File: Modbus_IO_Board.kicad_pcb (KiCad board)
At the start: 2 copper layers, 71.5 x 45 mm, 74 parts, among them IC1 ATMEGA328PB-AN, IC2 TPS7B6933QDCYRQ1, IC3 MAX3072EASA+, IC4 SN74LVC2G14DBVRG4, IC5 LTV-206, J1 Conn_01x06_Male, J2 2.54mm pitch Terminal Block, J3 282834-5, U1 PSM712-LF-T7, Y1 7.37MHz

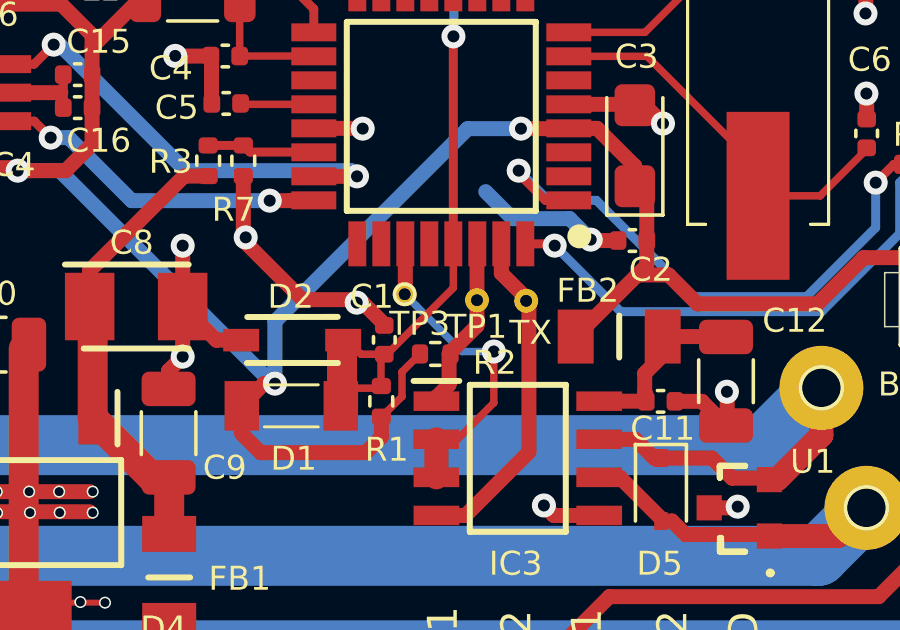
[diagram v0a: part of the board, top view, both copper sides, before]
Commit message: Review Pending
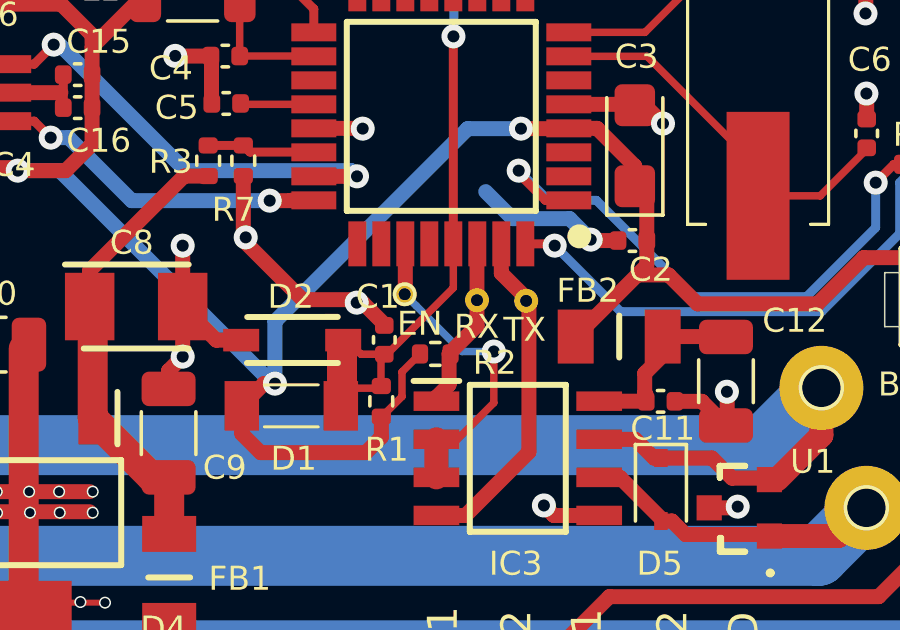
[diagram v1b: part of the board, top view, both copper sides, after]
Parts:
- renumbered TP3 to EN, TP1 to RX
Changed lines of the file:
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@@
     (32 B.Adhes user)
     (33 F.Adhes user)
-    (34 B.Paste user)
+    (34 B.Paste user hide)
     (35 F.Paste user)
     (36 B.SilkS user)
@@
     (visible_elements 7FFDFFFF)
     (pcbplotparams
-      (layerselection 0x00030_7ffffffe)
+      (layerselection 0x3ffff_ffffffff)
       (usegerberextensions false)
       (usegerberattributes true)
@@
       (padsonsilk false)
       (subtractmaskfromsilk false)
-      (outputformat 3)
+      (outputformat 1)
       (mirror false)
       (drillshape 0)
@@
     (tags "test point SMD pad")
     (attr virtual)
-    (fp_text reference TP1 (at -0.13 -0.66) (layer F.SilkS)
+    (fp_text reference RX (at -0.13 -0.66) (layer F.SilkS)
       (effects (font (size 0.8 0.8) (thickness 0.1)))
     )
@@
       (effects (font (size 1 1) (thickness 0.15)))
     )
-    (fp_text user TX (at -0.8 -0.0592) (layer F.SilkS)
+    (fp_text user TX (at -0.6 0.0408) (layer F.SilkS)
       (effects (font (size 0.8 0.8) (thickness 0.1)))
     )
@@
     (tags capacitor)
     (attr smd)
-    (fp_text reference C1 (at 1.44 -0.42 180) (layer F.SilkS)
+    (fp_text reference C1 (at 1.44 -0.22 180) (layer F.SilkS)
       (effects (font (size 0.8 0.8) (thickness 0.1)))
     )
@@
     (tags "test point SMD pad")
     (attr virtual)
-    (fp_text reference TP3 (at -0.5 -0.98 180) (layer F.SilkS)
-      (effects (font (size 0.8 0.8) (thickness 0.1)))
-    )
+    (fp_text reference EN (at -0.5 -0.98 180) (layer F.SilkS)
+      (effects (font (size 0.8 0.8) (thickness 0.1)))
+    )
